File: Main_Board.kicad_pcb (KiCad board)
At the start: 2 copper layers, 90 x 90 mm, 62 parts, among them J1 DAC_12-bits, J2 Bias_Header, J3 Measurement_Header, Q1 Q_PNP_BCE, Q2 Q_NPN_BCE, U1 AD667, U2 LF356

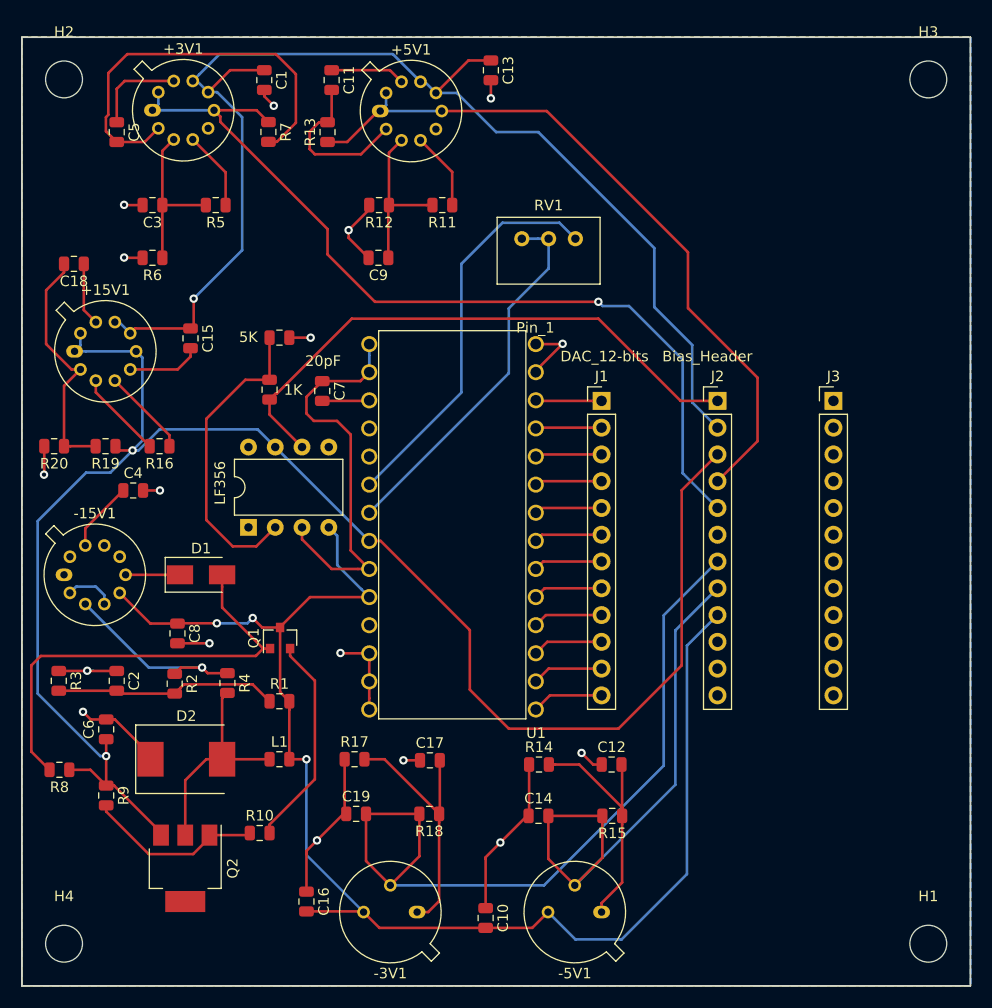
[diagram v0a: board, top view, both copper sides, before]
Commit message: Fin
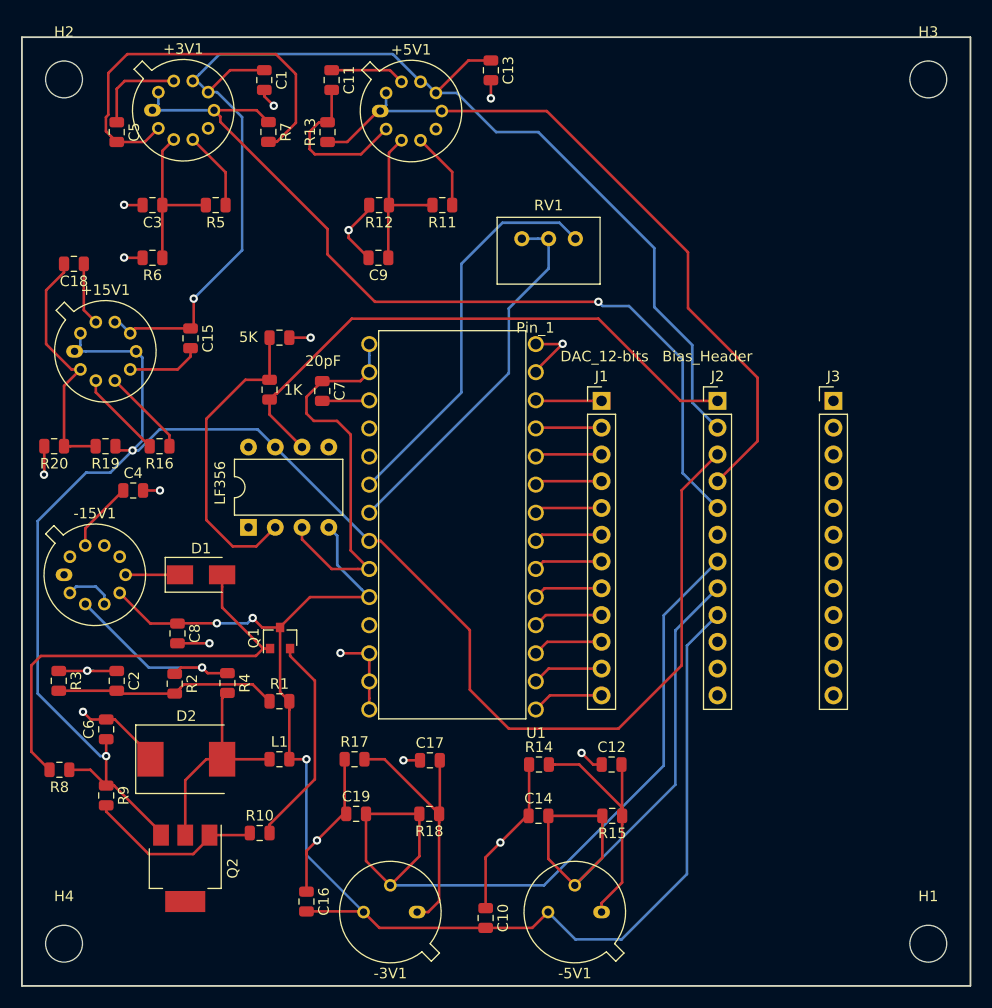
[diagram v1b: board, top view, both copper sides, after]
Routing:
- removed copper zone on B.Cu, net GND
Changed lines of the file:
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@@
   (segment (start 35.5 115.375) (end 36.056237 114.818763) (width 0.25) (layer F.Cu) (net 50))
   (segment (start 36.056237 114.818763) (end 36.181237 114.818763) (width 0.25) (layer F.Cu) (net 50))
-  (zone (net 1) (net_name GND) (layer B.Cu) (hatch edge 0.508)
-    (connect_pads (clearance 0.508))
-    (min_thickness 0.254)
-    (fill (arc_segments 32) (thermal_gap 0.508) (thermal_bridge_width 0.508))
-    (polygon
-      (pts
-        (xy 12 81) (xy 102 81) (xy 102 171) (xy 12 171)
-      )
-    )
-  )
-  (zone (net 1) (net_name GND) (layer B.Cu) (hatch edge 0.508)
-    (connect_pads (clearance 0.508))
-    (min_thickness 0.254)
-    (fill (arc_segments 32) (thermal_gap 0.508) (thermal_bridge_width 0.508))
-    (polygon
-      (pts
-        (xy 12 81) (xy 102 81) (xy 102 171) (xy 12 171)
-      )
-    )
-  )
-  (zone (net 1) (net_name GND) (layer B.Cu) (hatch edge 0.508)
-    (connect_pads (clearance 0.508))
-    (min_thickness 0.254)
-    (fill (arc_segments 32) (thermal_gap 0.508) (thermal_bridge_width 0.508))
-    (polygon
-      (pts
-        (xy 12 81) (xy 102 81) (xy 102 171) (xy 12 171)
-      )
-    )
-  )
-  (zone (net 1) (net_name GND) (layer B.Cu) (hatch edge 0.508)
-    (connect_pads (clearance 0.508))
-    (min_thickness 0.254)
-    (fill (arc_segments 32) (thermal_gap 0.508) (thermal_bridge_width 0.508))
-    (polygon
-      (pts
-        (xy 102.043 171.043) (xy 12 171.043) (xy 12 81) (xy 102.043 81)
-      )
-    )
-  )
 )
